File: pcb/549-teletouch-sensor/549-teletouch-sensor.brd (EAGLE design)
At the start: 75.9 x 76.2 mm, 87 parts, among them J1 RASPBERRYPI-40-PIN-GPIO_PTH, J2 RASPBERRYPI-40-PIN-GPIO_PTH

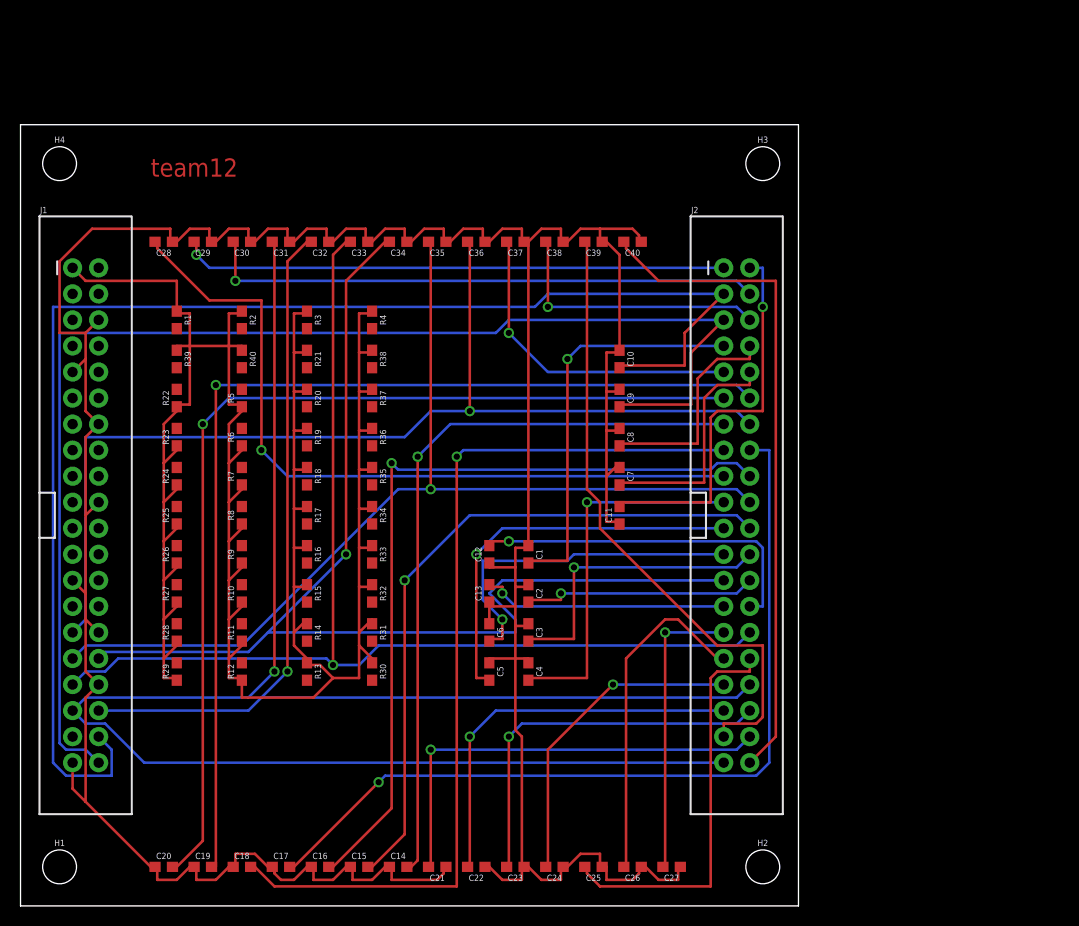
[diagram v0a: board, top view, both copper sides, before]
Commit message: updated sensor pcb
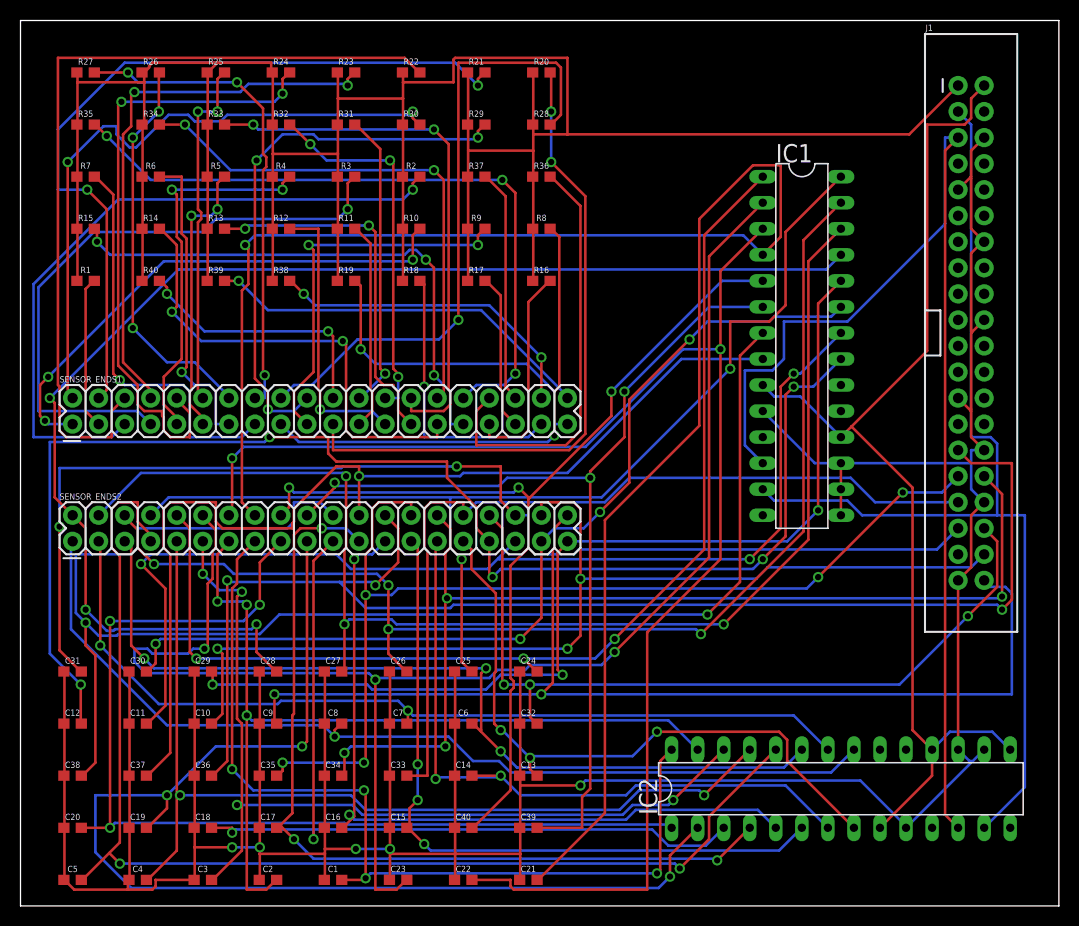
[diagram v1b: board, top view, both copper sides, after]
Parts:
- removed H1, H2, H3, H4: STAND-OFF, SparkFun-Hardware:STAND-OFF
- removed J2: RASPBERRYPI-40-PIN-GPIO_PTH, SparkFun-Connectors:2X20_SHROUDED
- added IC1, IC2: MCP23017SP, adafruit:DIL28-3
- added SENSOR_ENDS1, SENSOR_ENDS2: CONN_20X2, SparkFun-Connectors:2X20
- moved J1 88.2 mm to (92.7, 55.9)
- moved C38 70.1 mm to (5.08, 12.7), turned to 0 degrees
- moved C37 63.8 mm to (11.4, 12.7), turned to 0 degrees
- moved R28 61.0 mm to (50.8, 76.2), turned to 0 degrees
- moved R29 60.8 mm to (44.5, 76.2), turned to 0 degrees
- moved C40 59.5 mm to (43.2, 7.62), turned to 0 degrees
- moved C36 58.5 mm to (17.8, 12.7), turned to 0 degrees
- moved C39 57.5 mm to (49.5, 7.62), turned to 0 degrees
- moved C35 54.6 mm to (24.1, 12.7), turned to 0 degrees
- moved C10 54.0 mm to (17.8, 17.8), turned to 0 degrees
- moved R30 53.5 mm to (38.1, 76.2), turned to 0 degrees
- moved C34 52.5 mm to (30.5, 12.7), turned to 0 degrees
- moved C33 52.2 mm to (36.8, 12.7), turned to 0 degrees
- moved R27 51.6 mm to (6.35, 81.3), turned to 0 degrees
- moved C11 51.2 mm to (11.4, 17.8), turned to 0 degrees
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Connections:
- removed net GP41: J1.37
- removed net GP42: J1.7
- removed net GP43: J1.11
- removed net GP44: J1.12
- removed net GP45: J1.15
- removed net GP46: J1.16
- removed net GP47: J1.18
- removed net GP48: J1.22
- removed net GP49: J1.13
- removed net N$11: R10.2
- removed net N$12: R1.2
- removed net N$13: R2.2
- removed net N$14: R3.2
- removed net N$15: R4.2
- removed net N$16: R5.2
- removed net N$17: R6.2
- removed net N$18: R7.2
- removed net N$19: R8.2
- removed net N$20: R9.2
- removed net N$31: R20.2
- removed net N$32: R11.2
- removed net N$33: R12.2
- removed net N$34: R13.2
- removed net N$35: R14.2
- removed net N$36: R15.2
- removed net N$37: R16.2
- removed net N$38: R17.2
- removed net N$39: R18.2
- removed net N$40: R19.2
- removed net N$51: R30.2
- removed net N$52: R21.2
- removed net N$53: R22.2
- removed net N$54: R23.2
- removed net N$55: R24.2
- removed net N$56: R25.2
- removed net N$57: R26.2
- removed net N$58: R27.2
- removed net N$59: R28.2
- removed net N$60: R29.2
- removed net N$71: R40.2
- removed net N$72: R31.2
- removed net N$73: R32.2
- removed net N$74: R33.2
- removed net N$75: R34.2
- removed net N$76: R35.2
- removed net N$77: R36.2
- removed net N$78: R37.2
- removed net N$79: R38.2
- removed net N$80: R39.2
- new net S1: R10.2, SENSOR_ENDS1.1
- new net S10: R9.2, SENSOR_ENDS1.19
- new net S11: R20.2, SENSOR_ENDS1.21
- new net S12: R11.2, SENSOR_ENDS1.23
- new net S13: R12.2, SENSOR_ENDS1.25
- new net S14: R13.2, SENSOR_ENDS1.27
- new net S15: R14.2, SENSOR_ENDS1.29
- new net S16: R15.2, SENSOR_ENDS1.31
- new net S17: R16.2, SENSOR_ENDS1.33
- new net S18: R17.2, SENSOR_ENDS1.35
- new net S19: R18.2, SENSOR_ENDS1.37
- new net S2: R1.2, SENSOR_ENDS1.3
- new net S20: R19.2, SENSOR_ENDS1.39
- new net S21: R30.2, SENSOR_ENDS1.2
- new net S22: R21.2, SENSOR_ENDS1.4
- new net S23: R22.2, SENSOR_ENDS1.6
- new net S24: R23.2, SENSOR_ENDS1.8
- new net S25: R24.2, SENSOR_ENDS1.10
- new net S26: R25.2, SENSOR_ENDS1.12
- new net S27: R26.2, SENSOR_ENDS1.14
- new net S28: R27.2, SENSOR_ENDS1.16
- new net S29: R28.2, SENSOR_ENDS1.18
- new net S3: R2.2, SENSOR_ENDS1.5
- new net S30: R29.2, SENSOR_ENDS1.20
- new net S31: R40.2, SENSOR_ENDS1.22
- new net S32: R31.2, SENSOR_ENDS1.24
- new net S33: R32.2, SENSOR_ENDS1.26
- new net S34: R33.2, SENSOR_ENDS1.28
- new net S35: R34.2, SENSOR_ENDS1.30
- new net S36: R35.2, SENSOR_ENDS1.32
- new net S37: R36.2, SENSOR_ENDS1.34
- new net S38: R37.2, SENSOR_ENDS1.36
- new net S39: R38.2, SENSOR_ENDS1.38
- new net S4: R3.2, SENSOR_ENDS1.7
- new net S40: R39.2, SENSOR_ENDS1.40
- new net S5: R4.2, SENSOR_ENDS1.9
- new net S6: R5.2, SENSOR_ENDS1.11
- new net S7: R6.2, SENSOR_ENDS1.13
- new net S8: R7.2, SENSOR_ENDS1.15
- new net S9: R8.2, SENSOR_ENDS1.17
- net GND: now also IC1.10, IC1.15, IC1.16, IC1.17, IC2.10, IC2.16, IC2.17
- net GP1: now also IC2.21, SENSOR_ENDS2.1; no longer J2.8
- net GP10: now also IC2.2, SENSOR_ENDS2.19; no longer J2.12
- net GP11: now also IC2.3, SENSOR_ENDS2.21; no longer J2.15
- net GP12: now also IC2.4, SENSOR_ENDS2.23; no longer J2.16
- net GP13: now also IC2.5, SENSOR_ENDS2.25; no longer J2.18
- net GP14: now also IC2.6, SENSOR_ENDS2.27; no longer J2.22
- net GP15: now also IC2.7, SENSOR_ENDS2.29; no longer J2.13
- net GP16: now also IC2.8, SENSOR_ENDS2.31; no longer J2.27
- net GP17: now also IC1.21, SENSOR_ENDS2.33; no longer J2.28
- net GP18: now also IC1.22, SENSOR_ENDS2.35; no longer J2.2
- net GP19: now also IC1.23, SENSOR_ENDS2.37; no longer J2.4
- net GP2: now also IC2.22, SENSOR_ENDS2.3; no longer J2.10
- net GP20: now also IC1.24, SENSOR_ENDS2.39; no longer J2.1
- net GP21: now also IC1.25, SENSOR_ENDS2.2; no longer J2.17
- net GP22: now also IC1.26, SENSOR_ENDS2.4; no longer J2.29
- net GP23: now also IC1.27, SENSOR_ENDS2.6; no longer J2.31
- net GP24: now also IC1.28, SENSOR_ENDS2.8; no longer J2.32
- net GP25: now also IC1.1, SENSOR_ENDS2.10; no longer J2.33
- net GP26: now also IC1.2, SENSOR_ENDS2.12; no longer J2.36
- net GP27: now also IC1.3, SENSOR_ENDS2.14; no longer J2.35
- net GP28: now also IC1.4, SENSOR_ENDS2.16; no longer J2.38
- net GP29: now also IC1.5, SENSOR_ENDS2.18; no longer J2.40
- net GP3: now also IC2.23, SENSOR_ENDS2.5; no longer J2.23
- net GP30: now also IC1.6, SENSOR_ENDS2.20; no longer J2.37
- net GP31: now also IC1.7, SENSOR_ENDS2.22; no longer J2.6
- net GP32: now also IC1.8, SENSOR_ENDS2.24; no longer J2.9
- net GP33: now also SENSOR_ENDS2.26; no longer J2.14
- net GP34: now also SENSOR_ENDS2.28; no longer J2.20
- net GP35: now also SENSOR_ENDS2.30; no longer J2.25
- net GP36: now also SENSOR_ENDS2.32; no longer J2.30
- net GP37: now also SENSOR_ENDS2.34; no longer J2.34
- net GP38: now also SENSOR_ENDS2.36; no longer J2.39
- net GP39: now also SENSOR_ENDS2.38; no longer J2.3
- net GP4: now also IC2.24, SENSOR_ENDS2.7; no longer J2.21
- net GP40: now also SENSOR_ENDS2.40; no longer J2.5
- net GP5: now also IC2.25, SENSOR_ENDS2.9; no longer J2.19
- net GP6: now also IC2.26, SENSOR_ENDS2.11; no longer J2.24
- net GP7: now also IC2.27, SENSOR_ENDS2.13; no longer J2.26
- net GP8: now also IC2.28, SENSOR_ENDS2.15; no longer J2.7
- net GP9: now also IC2.1, SENSOR_ENDS2.17; no longer J2.11
- net SCL: now also IC1.12, IC2.12
- net SDA: now also IC1.13, IC2.13
- net VDD: now also IC1.18, IC1.9, IC2.15, IC2.18, IC2.9
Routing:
- net GP28: track 43.3 -> 169.6 mm
- net GP31: track 26.8 -> 144.7 mm, vias 1 -> 2
- net SCL: track 0.00 -> 115.4 mm
- net GP26: track 37.5 -> 145.0 mm, vias 1 -> 3
- net GP27: track 38.7 -> 144.7 mm, vias 1 -> 2
- net VDD: track 0.00 -> 105.5 mm
- net SDA: track 0.00 -> 100.8 mm
- net GP17: track 34.3 -> 133.6 mm, vias 1 -> 5
- net GP22: track 28.8 -> 125.9 mm, vias 1 -> 3
- net GP23: track 33.2 -> 117.3 mm, vias 0 -> 4
- net S23: track 0.00 -> 82.0 mm
- net GP4: track 38.7 -> 117.0 mm, vias 1 -> 2
- net GP25: track 31.4 -> 109.3 mm, vias 1 -> 3
- net S22: track 0.00 -> 76.3 mm, vias 0 -> 2
- net GP1: track 21.3 -> 93.4 mm, vias 0 -> 1
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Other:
- board size 75.9 x 76.2 mm -> 101.3 x 86.3 mm
- board text removed: "team12"
